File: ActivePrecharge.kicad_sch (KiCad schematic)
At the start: 52 parts, among them Con1 LED, IC1 1769205241, J1 Conn_01x03, J2 Conn_01x02, J3 Conn_01x02, Q1 IRLML0030, Q2 PMV35EPER, Q3 IRLML0030, U3 TLV9301xDCK, U4 TCMT1106

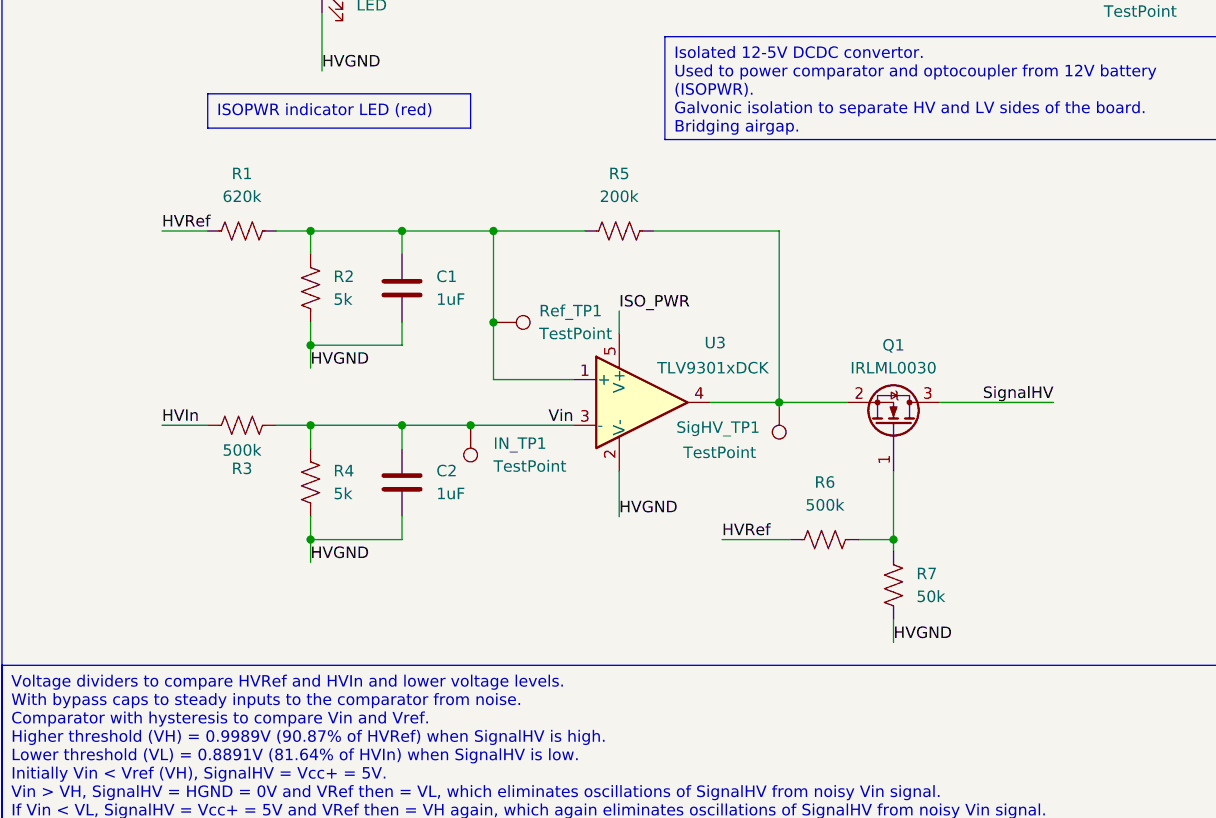
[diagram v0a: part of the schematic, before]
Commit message: finished for review
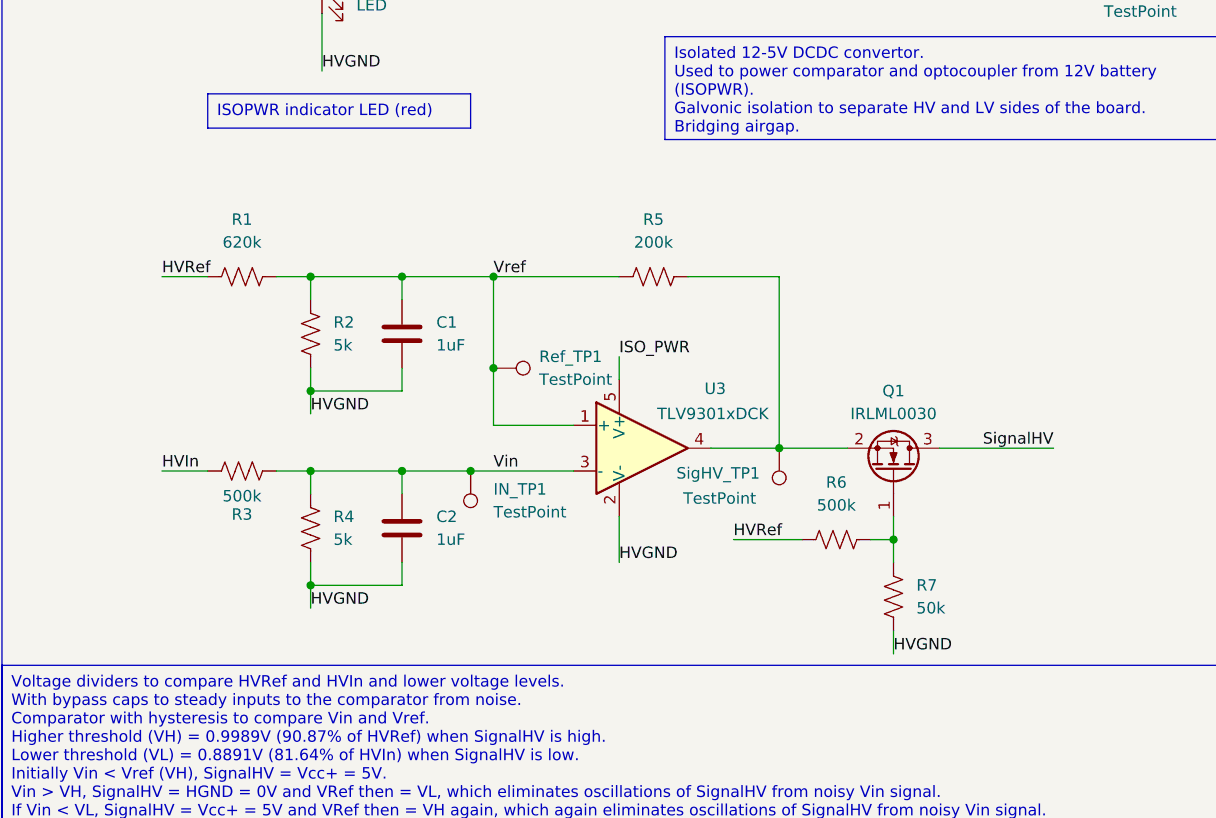
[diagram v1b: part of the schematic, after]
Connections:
- net HVGND: now also R7.1; no longer R7.2
- net Vref: now reaches C1.1, R1.2, R2.1, Ref_TP1.1, U3.1 (+)
- net Vref: now also R5.2; no longer R5.1
- net at Q1.2 (S), SigHV_TP1.1, U3.4: now also R5.1; no longer R5.2
- net at Q1.1 (G), R6.2: now also R7.2; no longer R7.1
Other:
- moved on the sheet: C1, C2, IN_TP1, Q1, R1, R2, R3, R4, R5, Ref_TP1, SigHV_TP1, U3
